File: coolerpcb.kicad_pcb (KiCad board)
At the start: 2 copper layers, 2 parts, among them J1 Conn_01x04_Socket, U1 TMP117xxDRV

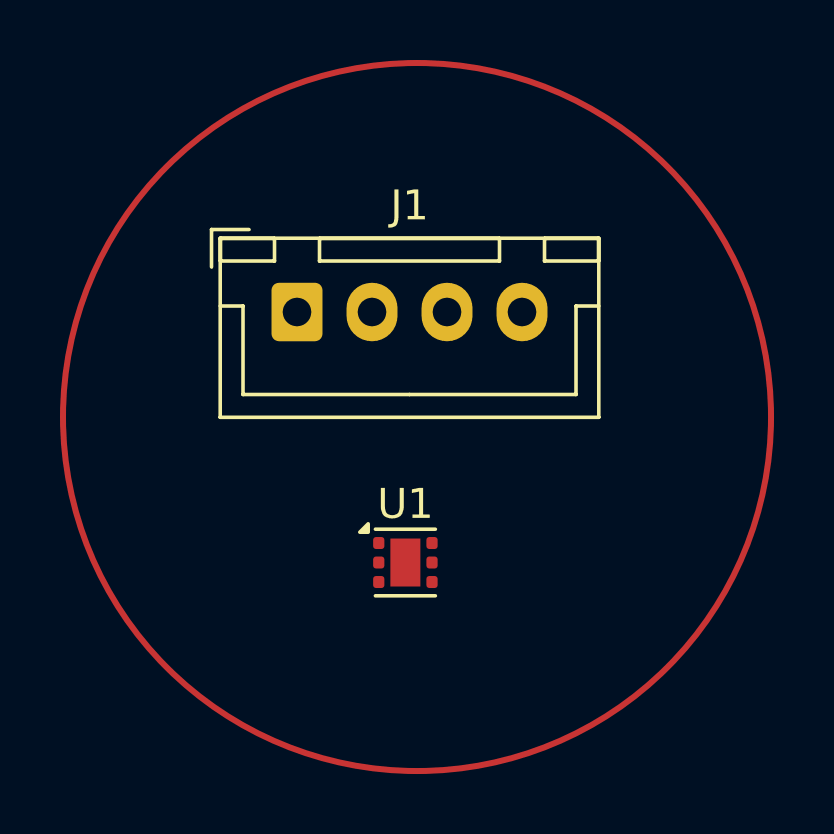
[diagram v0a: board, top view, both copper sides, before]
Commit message: 2/4
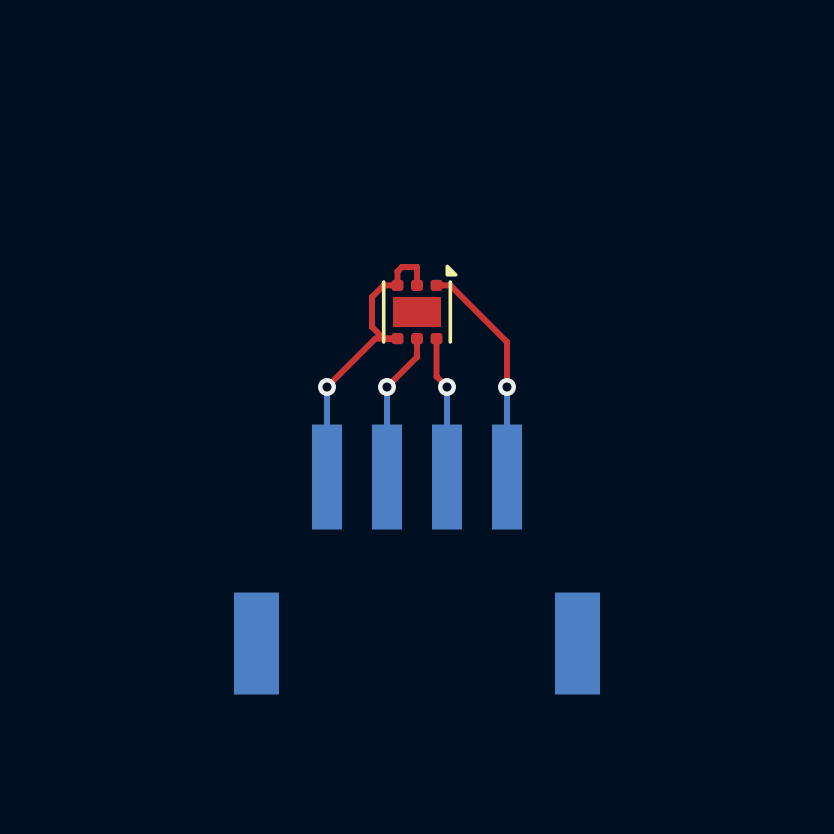
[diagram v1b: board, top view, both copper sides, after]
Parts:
- J1: value Conn_01x04_Socket -> S4B-PH-SM4-TB; footprint Connector_JST:JST_XH_B4B-XH-A_1x04_P2.50mm_Vertical -> S4B_PH_SM4_TB:JST_S4B-PH-SM4-TB; moved to B.Cu
- moved J1 9.17 mm to (59.0, 39.2), turned to 180 degrees
- moved U1 8.36 mm to (59.0, 31.0), turned to -90 degrees
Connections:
- J1 pad 1: GND -> Net-(U1-SCL)
- J1 pad 2: VCC -> Net-(U1-SDA)
- J1 pad 3: Net-(J1-Pin_3) -> VCC
- J1 pad 4: Net-(J1-Pin_4) -> GND
- U1 pad 1: Net-(J1-Pin_4) -> Net-(U1-SCL)
- U1 pad 6: Net-(J1-Pin_3) -> Net-(U1-SDA)
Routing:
- net GND: track 0.00 -> 10.8 mm, vias 0 -> 1
- net Net-(U1-SCL): track 0.00 -> 7.63 mm, vias 0 -> 1
- net VCC: track 0.00 -> 5.03 mm, vias 0 -> 1
- net Net-(U1-SDA): track 0.00 -> 4.76 mm, vias 0 -> 1
